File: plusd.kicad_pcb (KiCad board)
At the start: 2 copper layers, 99.1 x 87.6 mm, 52 parts, among them J1 Conn_02x17_Odd_Even, J2 ZX_Spectrum_Connector_GENERIC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, J3 Conn_02x13_Odd_Even, J4 Conn_01x03, SW1 SW_DPST_x2, SW2 SW_DIP_x02, U1 74LS06, U10 74LS27, U12 L7805, U2 AT28C256, U3 WD1772, U4 74LS00, U5 74LS126, U6 74LS175, U7 62256, U8 PAL20L8, U9 74LS374, Y1 8.000Mhz

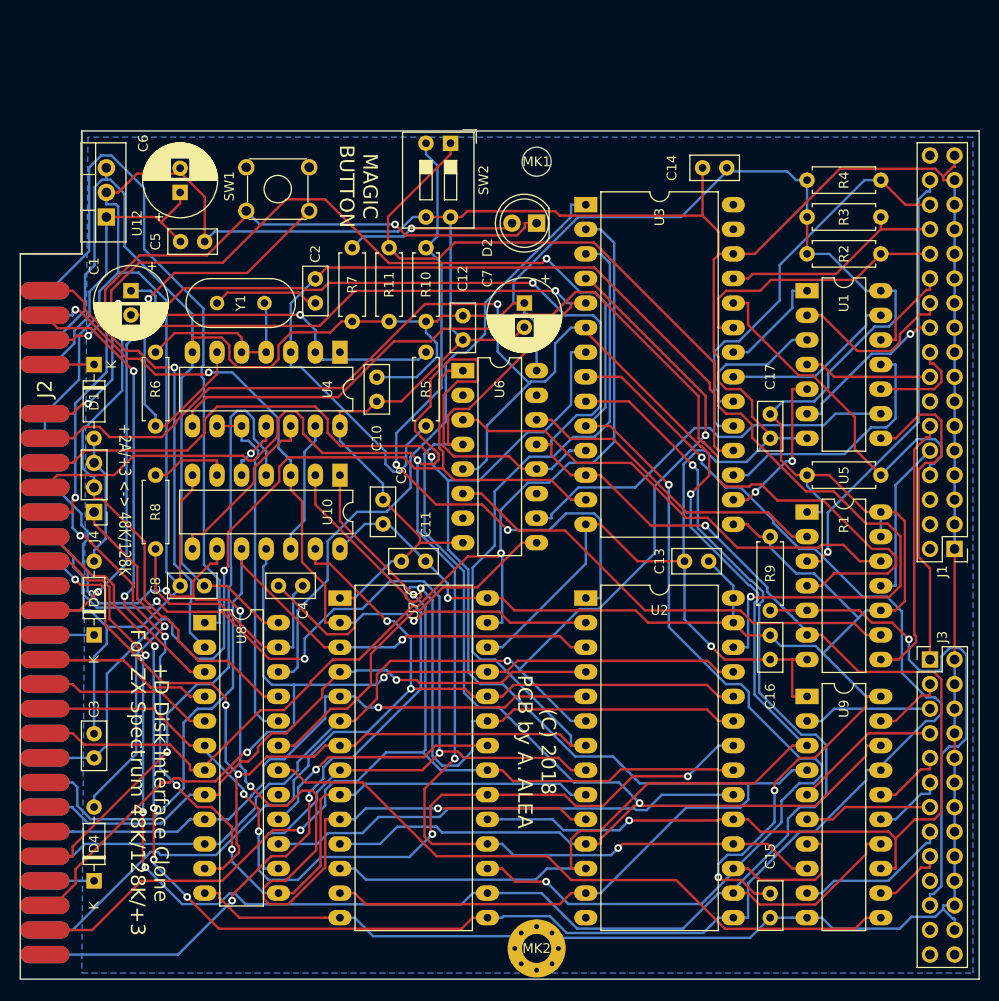
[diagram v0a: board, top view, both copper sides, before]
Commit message: ahora con joystick
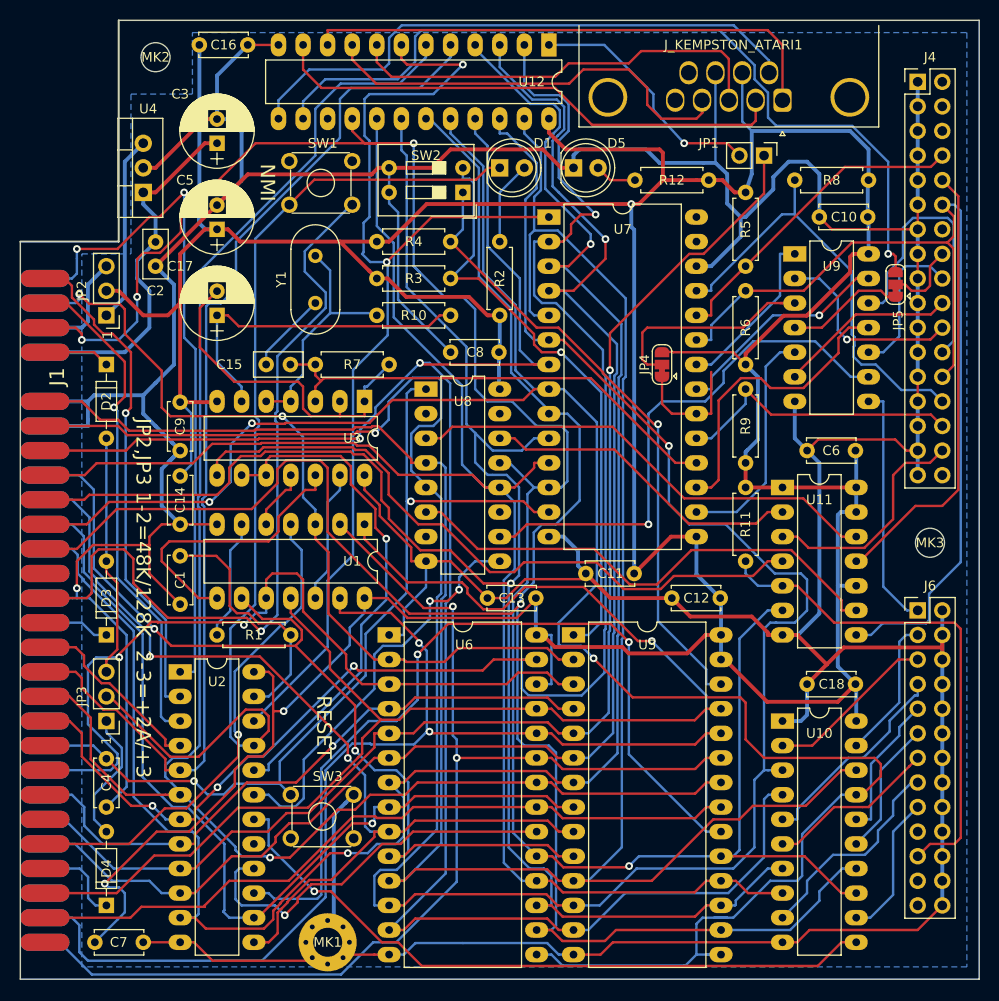
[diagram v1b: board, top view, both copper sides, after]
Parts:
- removed J2: ZX_Spectrum_Connector_GENERIC_SORTED, SINCLAIR:ZX_CONN
- removed J3: Conn_02x13_Odd_Even, Connector_PinHeader_2.54mm:PinHeader_2x13_P2.54mm_Vertical
- added C18: 100n, Capacitors_THT:C_Disc_D5.0mm_W2.5mm_P5.00mm, F.Cu at (116.8, 94.0)
- added D5: LED, LEDs:LED_D5.0mm, F.Cu at (92.7, 40.6)
- added J6: Conn_02x13_Odd_Even, Connector_PinHeader_2.54mm:PinHeader_2x13_P2.54mm_Vertical, F.Cu at (128.3, 86.4)
- added JP1: Jumper, Connector_PinHeader_2.54mm:PinHeader_1x02_P2.54mm_Vertical, F.Cu at (112.4, 39.4)
- added JP2: Conn_01x03, Connector_PinHeader_2.54mm:PinHeader_1x03_P2.54mm_Vertical, F.Cu at (44.5, 55.9)
- added JP3: Conn_01x03, Connector_PinHeader_2.54mm:PinHeader_1x03_P2.54mm_Vertical, F.Cu at (44.5, 97.8)
- added JP4: Jumper_NC_Dual, Jumper:SolderJumper-3_P1.3mm_Bridged12_RoundedPad1.0x1.5mm, F.Cu at (101.9, 61.0)
- added JP5: Jumper_NC_Dual, Jumper:SolderJumper-3_P1.3mm_Bridged12_RoundedPad1.0x1.5mm, F.Cu at (126.0, 52.7)
- added J_KEMPSTON_ATARI1: DB9_Male, Connector_Dsub:DSUB-9_Male_Horizontal_P2.77x2.84mm_EdgePinOffset4.94mm_Housed_MountingHolesOffset7.48mm, F.Cu at (114.3, 33.7)
- added MK3: Mounting_Hole, MountingHole:MountingHole_3mm, F.Cu at (129.5, 79.4)
- added R12: 2K2, Resistors_THT:R_Axial_DIN0207_L6.3mm_D2.5mm_P7.62mm_Horizontal, F.Cu at (99.1, 41.9)
- added SW3: SW_DPST_x2, Buttons_Switches_THT:SW_TH_Tactile_Omron_B3F-10xx, F.Cu at (63.5, 105.4)
- added U11: 74LS126, Housings_DIP:DIP-14_W7.62mm_LongPads, F.Cu at (114.3, 73.7)
- C1: value 100u -> 100p; footprint Capacitor_THT:CP_Radial_D7.5mm_P2.50mm -> Capacitors_THT:C_Disc_D5.0mm_W2.5mm_P5.00mm
- C10, C11, C12, C13, C14, C16, C8, C9: footprint Capacitor_THT:C_Disc_D5.0mm_W2.5mm_P2.50mm -> Capacitors_THT:C_Disc_D5.0mm_W2.5mm_P5.00mm
- C15: value 100n -> 33p; footprint Capacitor_THT:C_Disc_D5.0mm_W2.5mm_P2.50mm -> Capacitors_THT:C_Disc_D5.0mm_W2.5mm_P2.50mm
- C17, C3: value 100n -> 100u/16 V; footprint Capacitor_THT:C_Disc_D5.0mm_W2.5mm_P2.50mm -> Capacitors_THT:CP_Radial_D7.5mm_P2.50mm
- C2: value 33p -> 10n; footprint Capacitor_THT:C_Disc_D5.0mm_W2.5mm_P2.50mm -> Capacitors_THT:C_Disc_D5.0mm_W2.5mm_P2.50mm
- C4: value 100p -> 100n; footprint Capacitor_THT:C_Disc_D5.0mm_W2.5mm_P2.50mm -> Capacitors_THT:C_Disc_D5.0mm_W2.5mm_P5.00mm
- C5: value 10n -> 100u/16 V; footprint Capacitor_THT:C_Disc_D5.0mm_W2.5mm_P2.50mm -> Capacitors_THT:CP_Radial_D7.5mm_P2.50mm
- C6, C7: value 100u -> 100n; footprint Capacitor_THT:CP_Radial_D7.5mm_P2.50mm -> Capacitors_THT:C_Disc_D5.0mm_W2.5mm_P5.00mm
- D1: value 1N4148 -> LED; footprint Diode_THT:D_DO-35_SOD27_P7.62mm_Horizontal -> LEDs:LED_D5.0mm
- D2: value LED -> 1N4148; footprint LED_THT:LED_D5.0mm -> Diodes_THT:D_DO-35_SOD27_P7.62mm_Horizontal
- D3, D4: footprint Diode_THT:D_DO-35_SOD27_P7.62mm_Horizontal -> Diodes_THT:D_DO-35_SOD27_P7.62mm_Horizontal
- J1: value Conn_02x17_Odd_Even -> ZX_Spectrum_Connector_GENERIC_SORTED; footprint Connector_PinHeader_2.54mm:PinHeader_2x17_P2.54mm_Vertical -> SINCLAIR:ZX_CONN
- J4: value Conn_01x03 -> Conn_02x17_Odd_Even; footprint Connector_PinHeader_2.54mm:PinHeader_1x03_P2.54mm_Vertical -> Connector_PinHeader_2.54mm:PinHeader_2x17_P2.54mm_Vertical
- R1: value 470 -> 270; footprint Resistor_THT:R_Axial_DIN0207_L6.3mm_D2.5mm_P7.62mm_Horizontal -> Resistors_THT:R_Axial_DIN0207_L6.3mm_D2.5mm_P7.62mm_Horizontal
- R10, R11: value 10K -> 2K2; footprint Resistor_THT:R_Axial_DIN0207_L6.3mm_D2.5mm_P7.62mm_Horizontal -> Resistors_THT:R_Axial_DIN0207_L6.3mm_D2.5mm_P7.62mm_Horizontal
- R2: value 470 -> 2K2; footprint Resistor_THT:R_Axial_DIN0207_L6.3mm_D2.5mm_P7.62mm_Horizontal -> Resistors_THT:R_Axial_DIN0207_L6.3mm_D2.5mm_P7.62mm_Horizontal
- R3, R4: value 470 -> 10K; footprint Resistor_THT:R_Axial_DIN0207_L6.3mm_D2.5mm_P7.62mm_Horizontal -> Resistors_THT:R_Axial_DIN0207_L6.3mm_D2.5mm_P7.62mm_Horizontal
- R5, R6, R9: value 2K2 -> 470; footprint Resistor_THT:R_Axial_DIN0207_L6.3mm_D2.5mm_P7.62mm_Horizontal -> Resistors_THT:R_Axial_DIN0207_L6.3mm_D2.5mm_P7.62mm_Horizontal
- R7: footprint Resistor_THT:R_Axial_DIN0207_L6.3mm_D2.5mm_P7.62mm_Horizontal -> Resistors_THT:R_Axial_DIN0207_L6.3mm_D2.5mm_P7.62mm_Horizontal
- R8: value 270 -> 470; footprint Resistor_THT:R_Axial_DIN0207_L6.3mm_D2.5mm_P7.62mm_Horizontal -> Resistors_THT:R_Axial_DIN0207_L6.3mm_D2.5mm_P7.62mm_Horizontal
- SW1: footprint Button_Switch_THT:SW_TH_Tactile_Omron_B3F-10xx -> Buttons_Switches_THT:SW_TH_Tactile_Omron_B3F-10xx
- U1: value 74LS06 -> 74LS27; footprint Package_DIP:DIP-14_W7.62mm_LongPads -> Housings_DIP:DIP-14_W7.62mm_LongPads
- U10: value 74LS27 -> 74LS374; footprint Package_DIP:DIP-14_W7.62mm_LongPads -> Housings_DIP:DIP-20_W7.62mm_LongPads
- U12: value L7805 -> GAL22V10; footprint Package_TO_SOT_THT:TO-220-3_Vertical -> Housings_DIP:DIP-24_W7.62mm_LongPads
- U2: value AT28C256 -> PAL20L8; footprint Package_DIP:DIP-28_W15.24mm_LongPads -> Housings_DIP:DIP-24_W7.62mm_LongPads
- U3: value WD1772 -> 74LS00; footprint Package_DIP:DIP-28_W15.24mm_LongPads -> Housings_DIP:DIP-14_W7.62mm_LongPads
- U4: value 74LS00 -> L7805; footprint Package_DIP:DIP-14_W7.62mm_LongPads -> TO_SOT_Packages_THT:TO-220-3_Vertical
- U5: value 74LS126 -> AT28C256; footprint Package_DIP:DIP-14_W7.62mm_LongPads -> Housings_DIP:DIP-28_W15.24mm_LongPads
- U6: value 74LS175 -> 6264; footprint Package_DIP:DIP-16_W7.62mm_LongPads -> Housings_DIP:DIP-28_W15.24mm_LongPads
- U7: value 62256 -> WD1772; footprint Package_DIP:DIP-28_W15.24mm_LongPads -> Housings_DIP:DIP-28_W15.24mm_LongPads
- U8: value PAL20L8 -> 74LS175; footprint Package_DIP:DIP-24_W7.62mm_LongPads -> Housings_DIP:DIP-16_W7.62mm_LongPads
- U9: value 74LS374 -> 74LS06; footprint Package_DIP:DIP-20_W7.62mm_LongPads -> Housings_DIP:DIP-14_W7.62mm_LongPads
- Y1: footprint Crystal:Crystal_HC18-U_Vertical -> Crystals:Crystal_HC49-U_Vertical
- moved J4 96.0 mm to (128.3, 31.8), turned to 0 degrees
- moved J1 94.0 mm to (38.1, 77.5), turned to 270 degrees
- moved C16 83.3 mm to (59.1, 27.9), turned to 180 degrees
- moved C15 77.3 mm to (61.0, 61.0), turned to 0 degrees
- moved C7 76.9 mm to (48.3, 120.7), turned to 180 degrees
- moved R8 76.2 mm to (115.6, 41.9), turned to 0 degrees
- moved C6 70.0 mm to (116.8, 69.8), turned to 0 degrees
- moved C14 65.3 mm to (52.1, 77.5), turned to 90 degrees
- moved R1 63.2 mm to (63.5, 88.9)
- moved C3 62.3 mm to (55.9, 38.1), turned to 90 degrees
- moved R6 61.3 mm to (110.5, 53.3)
- moved C17 58.5 mm to (55.9, 55.9)
- moved U10 52.3 mm to (114.3, 97.8), turned to 0 degrees
- moved U1 51.7 mm to (71.1, 77.5), turned to 270 degrees
- moved C10 49.5 mm to (118.1, 45.7), turned to 0 degrees
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- renumbered MK2 to MK1, MK1 to MK2
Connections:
- C1 pad 1: Net-(C1-Pad1) -> GND
- C15 pad 1: GND -> Net-(C15-Pad1)
- C15 pad 2: +5V -> Net-(C15-Pad2)
- C17 pad 1: GND -> Net-(C17-Pad1)
- C17 pad 2: +5V -> Net-(C17-Pad2)
- C2 pad 1: Net-(C2-Pad1) -> GND
- C2 pad 2: Net-(C2-Pad2) -> +9V
- C3 pad 1: GND -> +9V
- C3 pad 2: /RESET -> GND
- C4 pad 2: Net-(C4-Pad2) -> /RESET
- C5 pad 1: GND -> +5V
- C5 pad 2: +9V -> GND
- C6 pad 1: +9V -> GND
- C6 pad 2: GND -> +5V
- C7 pad 1: +5V -> GND
- C7 pad 2: GND -> +5V
- D1 pad 1: ZX_ROMOE1 -> Net-(D1-Pad1)
- D2 pad 1: Net-(D2-Pad1) -> ZX_ROMOE1
- D3 pad 2: Net-(D1-Pad2) -> Net-(D2-Pad2)
- J4 pad 1: Net-(D4-Pad2) -> GND
- J4 pad 2: Net-(D2-Pad1) -> (no net)
- J4 pad 3: Net-(D1-Pad2) -> GND
- R1 pad 1: Net-(J1-Pad8) -> Net-(C1-Pad2)
- R1 pad 2: +5V -> Net-(R1-Pad2)
- R10 pad 1: ROM_A14 -> Net-(R10-Pad1)
- R10 pad 2: +5V -> Net-(C17-Pad1)
- R11 pad 1: ROM_A13 -> Net-(J5-Pad11)
- R2 pad 1: Net-(J1-Pad26) -> Net-(D1-Pad2)
- R3 pad 1: Net-(J1-Pad28) -> ROM_A14
- R4 pad 1: Net-(J1-Pad30) -> ROM_A13
- R5 pad 1: Net-(C1-Pad2) -> /INDEX
- R5 pad 2: Net-(C2-Pad2) -> +5V
- R6 pad 1: Net-(R6-Pad1) -> /DS1
- R6 pad 2: Net-(C1-Pad1) -> +5V
- R7 pad 1: Net-(D2-Pad2) -> Net-(C17-Pad2)
- R7 pad 2: +5V -> Net-(C15-Pad2)
- R8 pad 1: Net-(C4-Pad2) -> Net-(J4-Pad28)
- R8 pad 2: Net-(R8-Pad2) -> +5V
- R9 pad 1: Net-(J3-Pad21) -> Net-(J4-Pad30)
- SW1 pad 2: Net-(D2-Pad1) -> Net-(D1-Pad1)
- U1 pad 1: Net-(U1-Pad1) -> /A10
- U1 pad 10: Net-(J1-Pad18) -> /A7
- U1 pad 11: Net-(U1-Pad11) -> /A8
- U1 pad 12: Net-(J1-Pad24) -> Net-(U1-Pad12)
- U1 pad 13: Net-(U1-Pad13) -> /A9
- U1 pad 2: Net-(J1-Pad22) -> /A11
- U1 pad 3: Net-(U1-Pad3) -> /A12
- U1 pad 4: Net-(J1-Pad16) -> /M1
- U1 pad 6: Net-(J1-Pad20) -> Net-(R1-Pad2)
- U1 pad 8: Net-(J3-Pad1) -> Net-(U1-Pad8)
- U1 pad 9: Net-(U1-Pad9) -> /A0
- U10 pad 1: /A10 -> GND
- U10 pad 10: /A7 -> GND
- U10 pad 11: /A8 -> PRN_CS
- U10 pad 12: Net-(U10-Pad12) -> Net-(J5-Pad9)
- U10 pad 13: /A9 -> /D7
- U10 pad 14: +5V -> /D4
- U10 pad 2: /A11 -> Net-(J5-Pad3)
- U10 pad 3: /A12 -> /D1
- U10 pad 4: /M1 -> /D2
- U10 pad 5: Net-(U10-Pad5) -> Net-(J5-Pad4)
- U10 pad 6: Net-(R8-Pad2) -> Net-(J5-Pad7)
- U10 pad 7: GND -> /D5
- U10 pad 8: Net-(U10-Pad8) -> /D6
- U10 pad 9: /A0 -> Net-(J5-Pad8)
- U12 pad 1: +9V -> Net-(JP1-Pad2)
- U12 pad 2: GND -> /WR
- U12 pad 3: +5V -> /A4
- U2 pad 1: ROM_A14 -> /A14
- U2 pad 10: /A0 -> /A4
- U2 pad 11: /D0 -> /A3
- U2 pad 12: /D1 -> GND
- U2 pad 13: /D2 -> /A1
- U2 pad 14: (no net) -> /A2
- U2 pad 15: /D3 -> ROM_CS
- U2 pad 16: /D4 -> RAM_CS
- U2 pad 17: /D5 -> (no net)
- U2 pad 18: /D6 -> PRN_CS
- U2 pad 19: /D7 -> DSK_CS
- U2 pad 2: /A12 -> /A15
- U2 pad 20: ROM_CS -> PRN_STR
- U2 pad 21: /A10 -> Net-(D1-Pad1)
- U2 pad 22: /RD -> FDC_CS
- U2 pad 23: /A11 -> Net-(C1-Pad2)
- U2 pad 24: /A9 -> +5V
- U2 pad 3: /A7 -> /A13
- U2 pad 4: /A6 -> /MREQ
- U2 pad 5: /A5 -> /IOREQ
- U2 pad 6: /A4 -> /RD
- U2 pad 7: /A3 -> /WR
- U2 pad 8: /A2 -> /A6
- U2 pad 9: /A1 -> /A5
- U3 pad 1: FDC_CS -> Net-(C17-Pad2)
- U3 pad 10: /D5 -> PRN_STR
- U3 pad 11: /D6 -> Net-(U1-Pad5)
- U3 pad 12: /D7 -> Net-(U1-Pad8)
- U3 pad 13: /RESET -> Net-(U1-Pad12)
- U3 pad 2: /WR -> Net-(C17-Pad2)
- U3 pad 3: /A3 -> Net-(C15-Pad2)
- U3 pad 4: /A4 -> Net-(R10-Pad1)
- U3 pad 5: /D0 -> Net-(R10-Pad1)
- U3 pad 6: /D1 -> Net-(C17-Pad1)
- U3 pad 7: /D2 -> +5V
- U3 pad 8: /D3 -> Net-(U11-Pad4)
- U3 pad 9: /D4 -> PRN_STR
- U4 pad 1: Net-(C1-Pad2) -> +9V
- U4 pad 2: Net-(C1-Pad2) -> GND
- U4 pad 3: Net-(C2-Pad2) -> Net-(JP2-Pad1)
- U5 pad 1: +5V -> ROM_A14
- U5 pad 10: +5V -> /A0
- U5 pad 11: /DS0 -> /D0
- U5 pad 12: Net-(U5-Pad12) -> /D1
- U5 pad 13: +5V -> /D2
- U5 pad 14: +5V -> GND
- U5 pad 2: Net-(U5-Pad2) -> /A12
- U5 pad 3: /XXX -> /A7
- U5 pad 4: Net-(U4-Pad8) -> /A6
- U5 pad 5: Net-(J3-Pad21) -> /A5
- U5 pad 6: /D7 -> /A4
- U5 pad 7: GND -> /A3
- U5 pad 8: /DS1 -> /A2
- U5 pad 9: Net-(U5-Pad9) -> /A1
- U6 pad 1: /RESET -> GND
- U6 pad 10: Net-(U1-Pad9) -> /A0
- U6 pad 11: (no net) -> /D0
- U6 pad 12: /D6 -> /D1
- U6 pad 13: /D7 -> /D2
- U6 pad 14: Net-(U5-Pad2) -> GND
- U6 pad 15: (no net) -> /D3
- U6 pad 16: +5V -> /D4
- U6 pad 2: (no net) -> /A12
- U6 pad 3: Net-(U5-Pad12) -> /A7
- U6 pad 4: /D0 -> /A6
- U6 pad 5: /D1 -> /A5
- U6 pad 6: Net-(U5-Pad9) -> /A4
- U6 pad 7: (no net) -> /A3
- U6 pad 8: GND -> /A2
- U6 pad 9: DSK_CS -> /A1
- U7 pad 1: GND -> FDC_CS
- U7 pad 10: /A0 -> /D5
- U7 pad 11: /D0 -> /D6
- U7 pad 12: /D1 -> /D7
- U7 pad 13: /D2 -> /RESET
- U7 pad 15: /D3 -> +5V
- U7 pad 16: /D4 -> Net-(U7-Pad16)
- U7 pad 17: /D5 -> Net-(U7-Pad17)
- U7 pad 18: /D6 -> Net-(C15-Pad2)
- U7 pad 19: /D7 -> Net-(J4-Pad30)
- U7 pad 2: /A12 -> /WR
- U7 pad 20: /RD -> Net-(JP4-Pad1)
- U7 pad 21: /A10 -> Net-(U7-Pad21)
- U7 pad 22: RAM_CS -> Net-(U7-Pad22)
- U7 pad 23: /A11 -> /DS1
- U7 pad 24: /A9 -> /INDEX
- U7 pad 25: /A8 -> Net-(J4-Pad28)
- U7 pad 27: /WR -> (no net)
- U7 pad 28: +5V -> (no net)
- U7 pad 3: /A7 -> /A3
- U7 pad 4: /A6 -> /A4
- U7 pad 5: /A5 -> /D0
- U7 pad 6: /A4 -> /D1
- U7 pad 7: /A3 -> /D2
- U7 pad 8: /A2 -> /D3
- U7 pad 9: /A1 -> /D4
- U8 pad 1: /A14 -> /RESET
- U8 pad 10: /A4 -> Net-(U8-Pad10)
- U8 pad 11: /A3 -> (no net)
- U8 pad 12: GND -> /D6
- U8 pad 13: /A1 -> /D7
- U8 pad 14: /A2 -> Net-(U11-Pad2)
- U8 pad 15: ROM_CS -> (no net)
- U8 pad 16: RAM_CS -> +5V
- U8 pad 2: /A15 -> (no net)
- U8 pad 3: /A13 -> Net-(U11-Pad12)
- U8 pad 4: /MREQ -> /D0
- U8 pad 5: /IOREQ -> /D1
- U8 pad 6: /RD -> Net-(U11-Pad9)
- U8 pad 7: /WR -> (no net)
- U8 pad 8: /A6 -> GND
- U8 pad 9: /A5 -> DSK_CS
- U9 pad 1: GND -> Net-(U7-Pad22)
- U9 pad 10: GND -> /DIR
- U9 pad 11: PRN_CS -> Net-(U7-Pad17)
- U9 pad 12: Net-(J3-Pad17) -> Net-(J4-Pad24)
- U9 pad 13: /D7 -> Net-(U7-Pad21)
- U9 pad 14: /D4 -> +5V
- U9 pad 2: Net-(J3-Pad5) -> Net-(J4-Pad22)
- U9 pad 3: /D1 -> Net-(JP4-Pad2)
- U9 pad 4: /D2 -> Net-(JP5-Pad1)
- U9 pad 5: Net-(J3-Pad7) -> Net-(U7-Pad16)
- U9 pad 6: Net-(J3-Pad13) -> /STEP
- U9 pad 7: /D5 -> GND
- U9 pad 8: /D6 -> Net-(J5-Pad1)
- U9 pad 9: Net-(J3-Pad15) -> Net-(U8-Pad10)
- Y1 pad 1: Net-(C2-Pad1) -> Net-(C15-Pad1)
- Y1 pad 2: Net-(R6-Pad1) -> Net-(R10-Pad1)
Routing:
- net +5V: track 389.3 -> 500.9 mm
- net Net-(D1-Pad1): track 0.00 -> 109.3 mm
- net Net-(D2-Pad1): track 106.5 -> 0.00 mm, vias 2 -> 0
- net Net-(U4-Pad8): track 105.7 -> 0.00 mm
- net /IOREQ: track 18.1 -> 111.9 mm
- net Net-(C2-Pad2): track 87.5 -> 0.00 mm
- net ALT_MOTOR_ON: track 0.00 -> 86.8 mm, vias 0 -> 1
- net /RD: track 91.4 -> 177.6 mm, vias 4 -> 1
- net GND: track 573.2 -> 658.0 mm
- net /DS1: track 27.7 -> 104.3 mm
- net Net-(U11-Pad4): track 0.00 -> 69.9 mm
- net /A5: track 65.1 -> 133.9 mm
- net J6-Fire: track 0.00 -> 60.1 mm
- net Net-(U8-Pad10): track 0.00 -> 55.4 mm, vias 0 -> 1
- net J1-Up: track 0.00 -> 54.9 mm
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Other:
- board size 99.1 x 87.6 mm -> 99.1 x 99.1 mm
- net class power added: clearance 0.2, trace_width 0.35, via_dia 0.8, via_drill 0.4
- board text added: "1"
- board text added: "Edicion para www.va-de-retro.com"
- board text added: "JP2,JP3 1-2=48K/128K 2-3=+2A/+3"
- board text added: "MGT's "+D" Clone Floppy Disk Interface For ZX Spectrum 48K/128K/+3"
- board text added: "NMI"
- board text added: "RESET"
- board text removed: "+2A/+3 <-> 48K/128K"
- board text removed: "+D Disk Interface Clone For ZX Spectrum 48K/128K/+3"
- board text removed: "MAGIC BUTTON"
